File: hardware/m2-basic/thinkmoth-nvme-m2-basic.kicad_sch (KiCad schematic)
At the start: 21 parts, among them J1 ExpressCard, J2 MDT180M03001, J3 TF-001B, U1 GL823K-HCY04

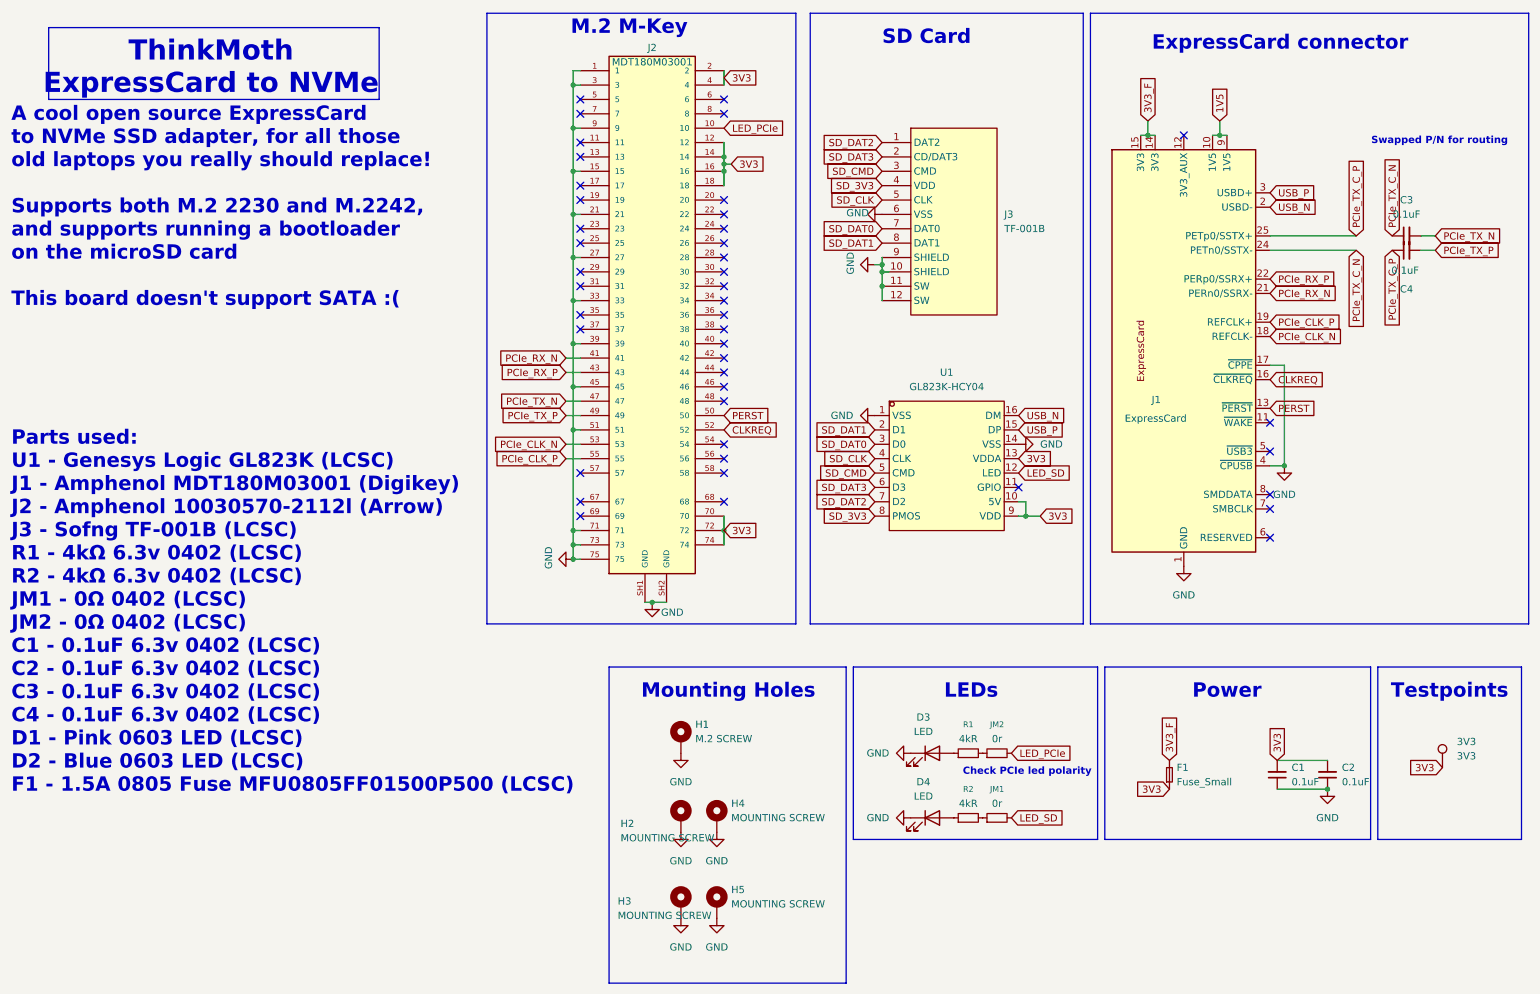
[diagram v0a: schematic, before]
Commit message: minor tweaks
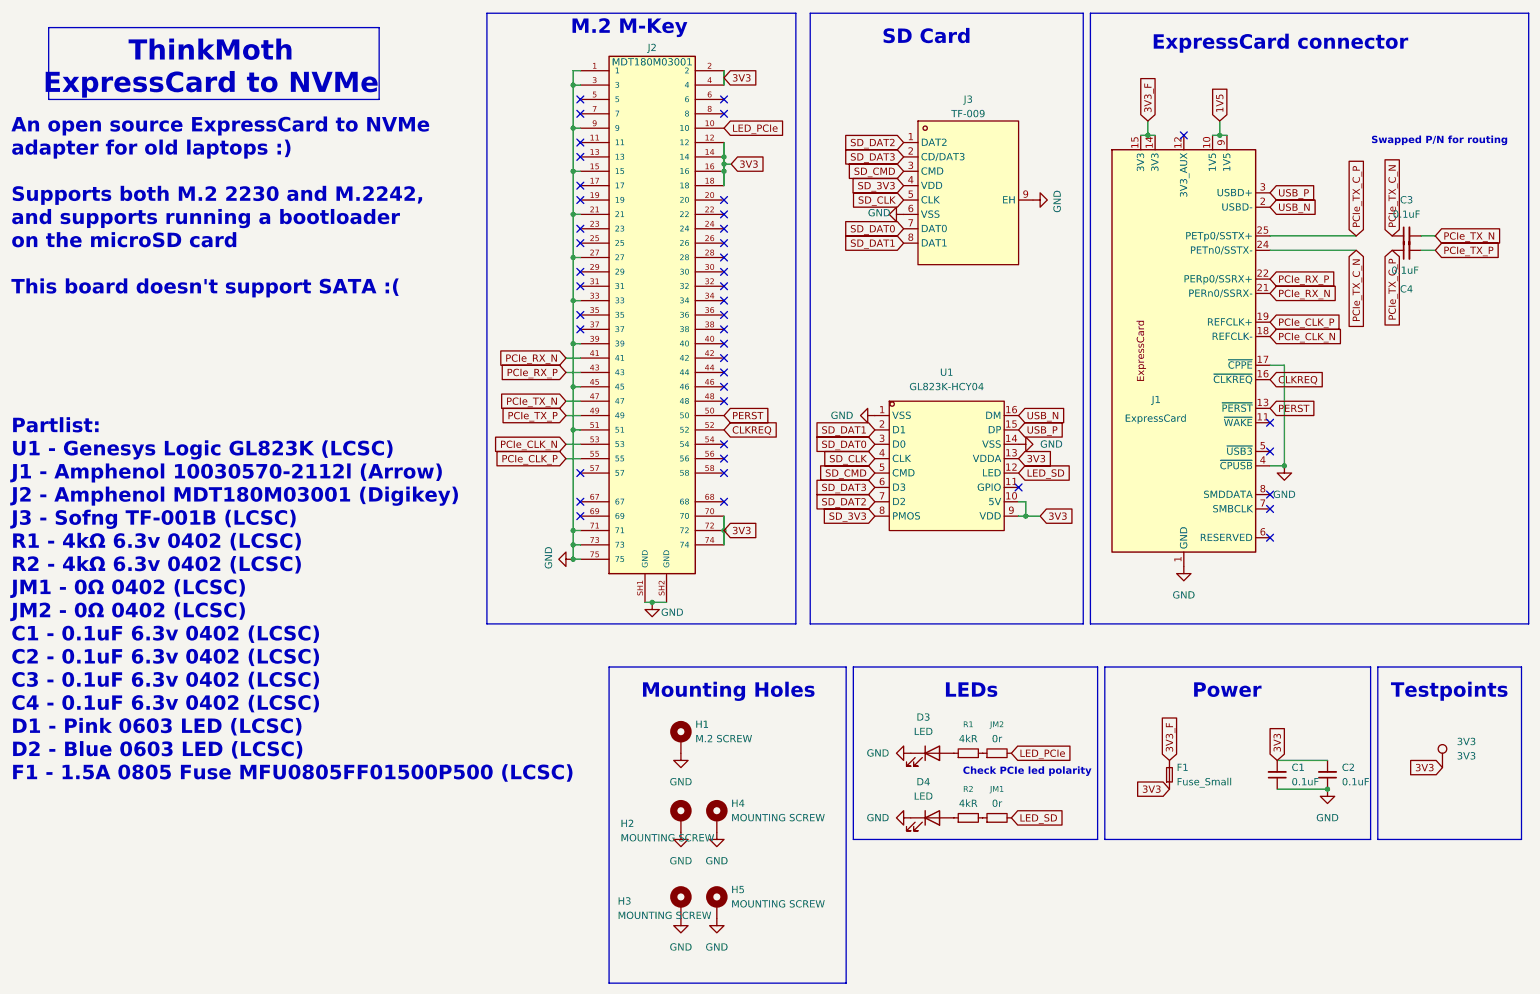
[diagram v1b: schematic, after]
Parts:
- removed J3: TF-001B, SOFNG-TF-001B:TF-SMD_TF-001B, symbol SOFNG-TF-001B:TF-001B
- added J3: TF-009, SOFNG-TF-009:TF-SMD_TF-009, symbol SOFNG-TF-009:TF-009
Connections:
- net GND: now also J3.6 (VSS), J3.9 (EH)
- net SD_3V3: now also J3.4 (VDD)
- net SD_CLK: now also J3.5 (CLK)
- net SD_CMD: now also J3.3 (CMD)
- net SD_DAT0: now also J3.7 (DAT0)
- net SD_DAT1: now also J3.8 (DAT1)
- net SD_DAT2: now also J3.1 (DAT2)
- net SD_DAT3: now also J3.2 (CD/DAT3)
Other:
- note added: "An open source ExpressCard to NVMe adapter for old laptops :) Supports both M.2 2230 and M.2242, and supports running a bootloader on the microSD card This board doesn't support SATA :( Partlist: U1 - Genesys Logic GL823K (LCSC) J1 - Amphenol 10030570-2112l (Arrow) J2 - Amphenol MDT180M03001 (Digikey) J3 - Sofng TF-001B (LCSC) R1 - 4kΩ 6.3v 0402 (LCSC) R2 - 4kΩ 6.3v 0402 (LCSC) JM1 - 0Ω 0402 (LCS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"
- note removed: "A cool open source ExpressCard to NVMe SSD adapter, for all those old laptops you really should replace! Supports both M.2 2230 and M.2242, and supports running a bootloader on the microSD card This board doesn't support SATA :( Parts used: U1 - Genesys Logic GL823K (LCSC) J1 - Amphenol MDT180M03001 (Digikey) J2 - Amphenol 10030570-2112l (Arrow) J3 - Sofng TF-001B (LCSC) R1 - 4kΩ 6.3v 0402 (LCSC)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"
